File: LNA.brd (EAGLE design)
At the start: 78.1 x 69.9 mm, 54 parts, among them IC1 LM4562, IC4 DCDC, Q1 nmos, Q2 JFET-DUAL, Q3 NPN, Q4 PNP, SW1 SW

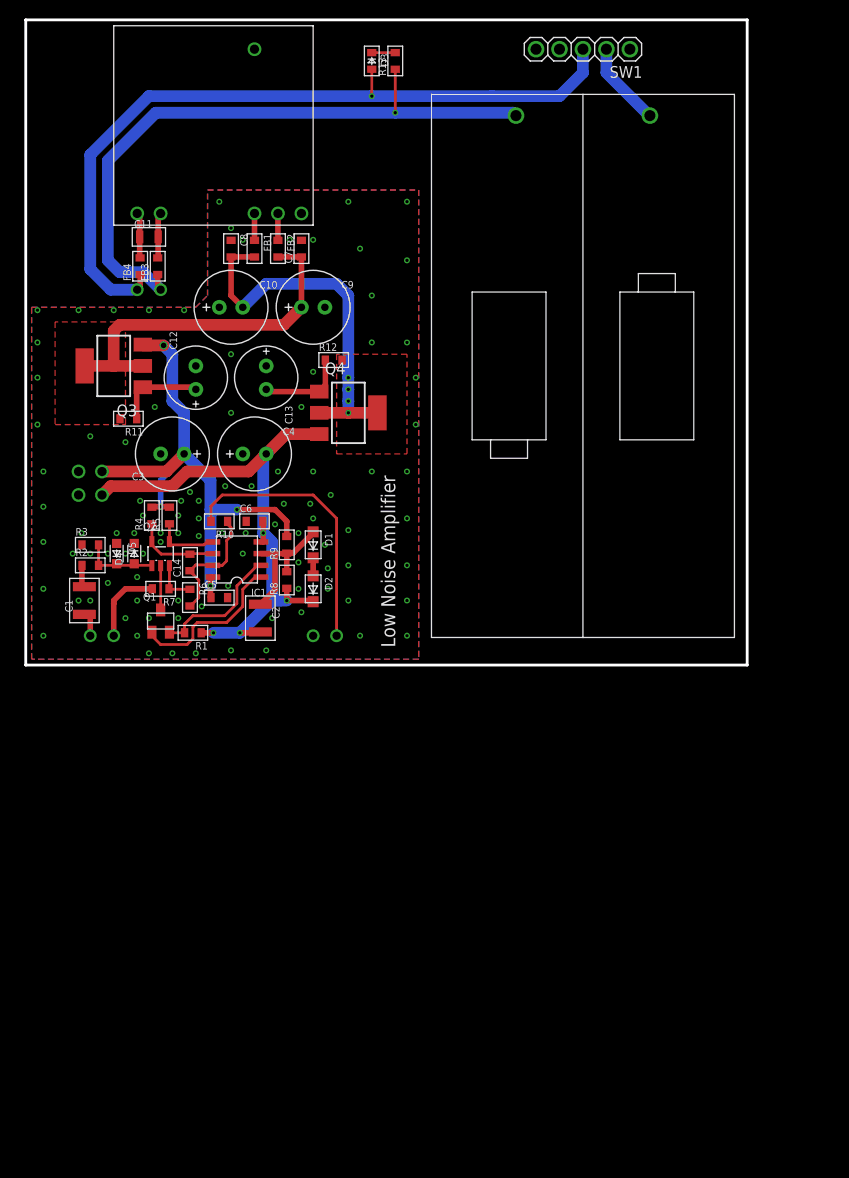
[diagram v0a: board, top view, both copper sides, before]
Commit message: 微修正
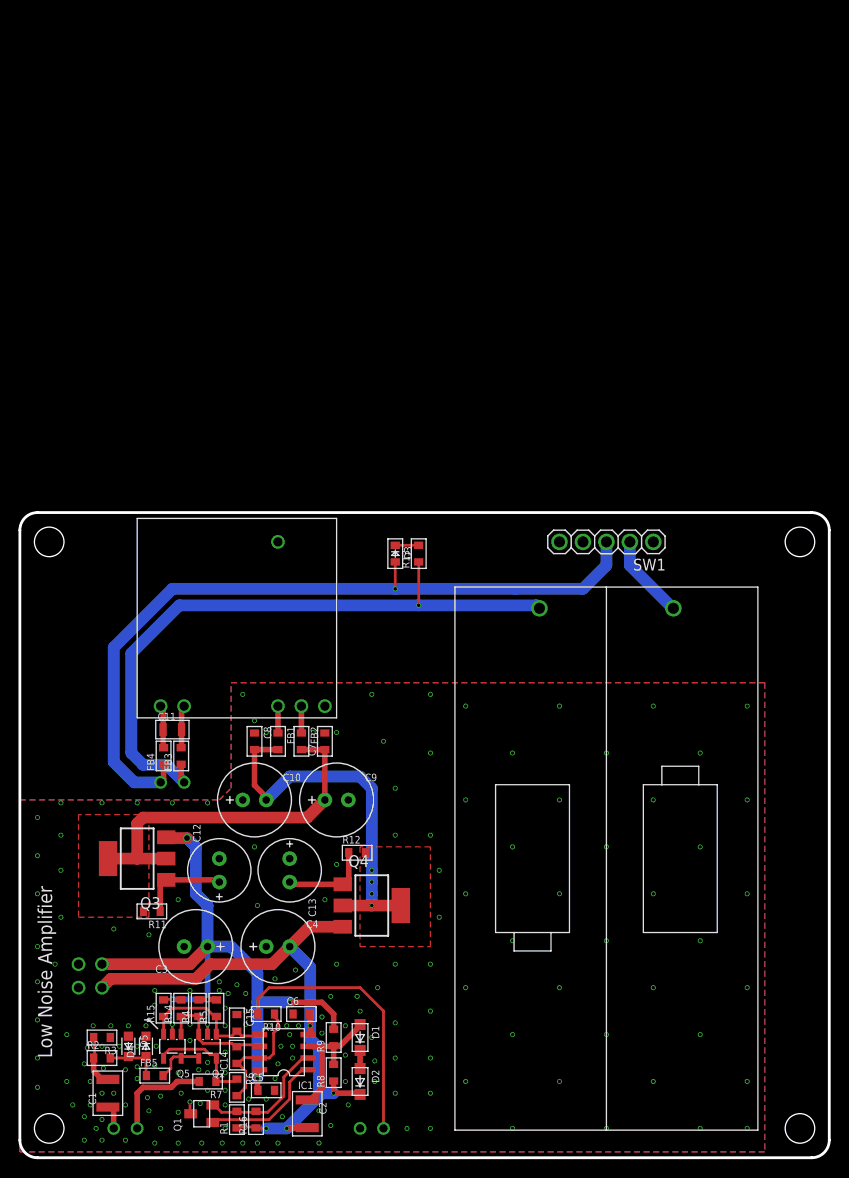
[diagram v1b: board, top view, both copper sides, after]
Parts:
- added C15: 10p, my_rcl:1608C
- added DR1, DR2, DR3, DR4: HOLE-3.2, my_connector:HOLE_3.2
- added FB5: FB, my_rcl:1608-FB
- added Q5: 2SK2145, my_ic:SOT23-5
- added R14, R15: 3.6k, my_rcl:1608
- added R16: DNP, my_rcl:1608
- C1: value 10u -> 3.3u
- C2: value 10u -> 22u
- D1, D2: value D -> BIAS
- D4, D5: value (none) -> CLAMP
- Q1: value nmos -> BS138
- Q2: value JFET-DUAL -> 2SK2145
- R1: value 1k -> 360
- moved C2 53.9 mm to (31.1, 4.13)
- moved C14 53.6 mm to (23.5, 10.5)
- moved C5 53.6 mm to (26.7, 6.67)
- moved C6 53.6 mm to (30.5, 14.9)
- moved D2 53.6 mm to (36.8, 7.62)
- moved IC1 53.6 mm to (28.6, 10.8)
- moved R10 53.6 mm to (26.7, 14.9)
- moved R7 53.6 mm to (20.3, 7.62)
- moved R8 53.6 mm to (34.0, 8.57)
- moved TP2 53.6 mm to (36.8, 2.54)
- moved TP3 53.6 mm to (39.4, 2.54)
- moved D1 53.6 mm to (36.8, 12.4)
- moved Q2 53.6 mm to (20.3, 11.4), turned to 180 degrees
- moved R4 53.6 mm to (19.4, 15.6)
- moved R5 53.6 mm to (21.3, 15.6)
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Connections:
- new net N$8: FB5.2, Q2.4, Q5.5
- net +5V: now also R14.2, R15.2
- net -5V: now also R16.1
- net GND: now also C15.1
- net N$2: now also R16.2
- net N$21: now also Q5.2
- net N$24: now also Q2.3, Q5.1, R14.1; no longer Q2.5
- net N$4: now also FB5.1; no longer Q2.1, R3.2
- net N$5: now also R3.2
- net N$7: now also C15.2, Q2.1, Q5.3, R15.1; no longer Q2.4
- net N$9: now also Q2.5, Q5.4; no longer Q2.3
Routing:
- net N$21: track 4.80 -> 17.9 mm, vias 0 -> 3
- net +5V: track 61.7 -> 71.5 mm, vias 4 -> 5
- net N$7: track 7.09 -> 15.6 mm
- net N$9: track 4.93 -> 11.9 mm
- net N$8: track 0.00 -> 5.58 mm
- net -5V: track 62.4 -> 67.5 mm
- net N$1: track 17.4 -> 13.9 mm
- net N$5: track 2.58 -> 5.63 mm
- net GND_IN: track 8.20 -> 10.7 mm
- net N$24: track 11.1 -> 13.5 mm
- net N$4: track 8.31 -> 6.82 mm
- net N$10: track 14.8 -> 15.3 mm
- added copper zone on layer 15, net GND
- added copper zone on layer 2, net GND
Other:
- board size 78.1 x 69.9 mm -> 87.6 x 69.9 mm
